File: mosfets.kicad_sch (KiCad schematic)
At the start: 25 parts, among them IC2 IRFR9014PBF, J4 Screw_Terminal_01x02, J5 Screw_Terminal_01x02, J6 Screw_Terminal_01x02, J7 Screw_Terminal_01x02, J8 Screw_Terminal_01x02, J9 Screw_Terminal_01x02, Q1 IRLML6244, Q2 IRLML6244, Q3 IRLML6244, Q4 IRLML6244, Q5 IRLML6244, Q6 IRLML6244

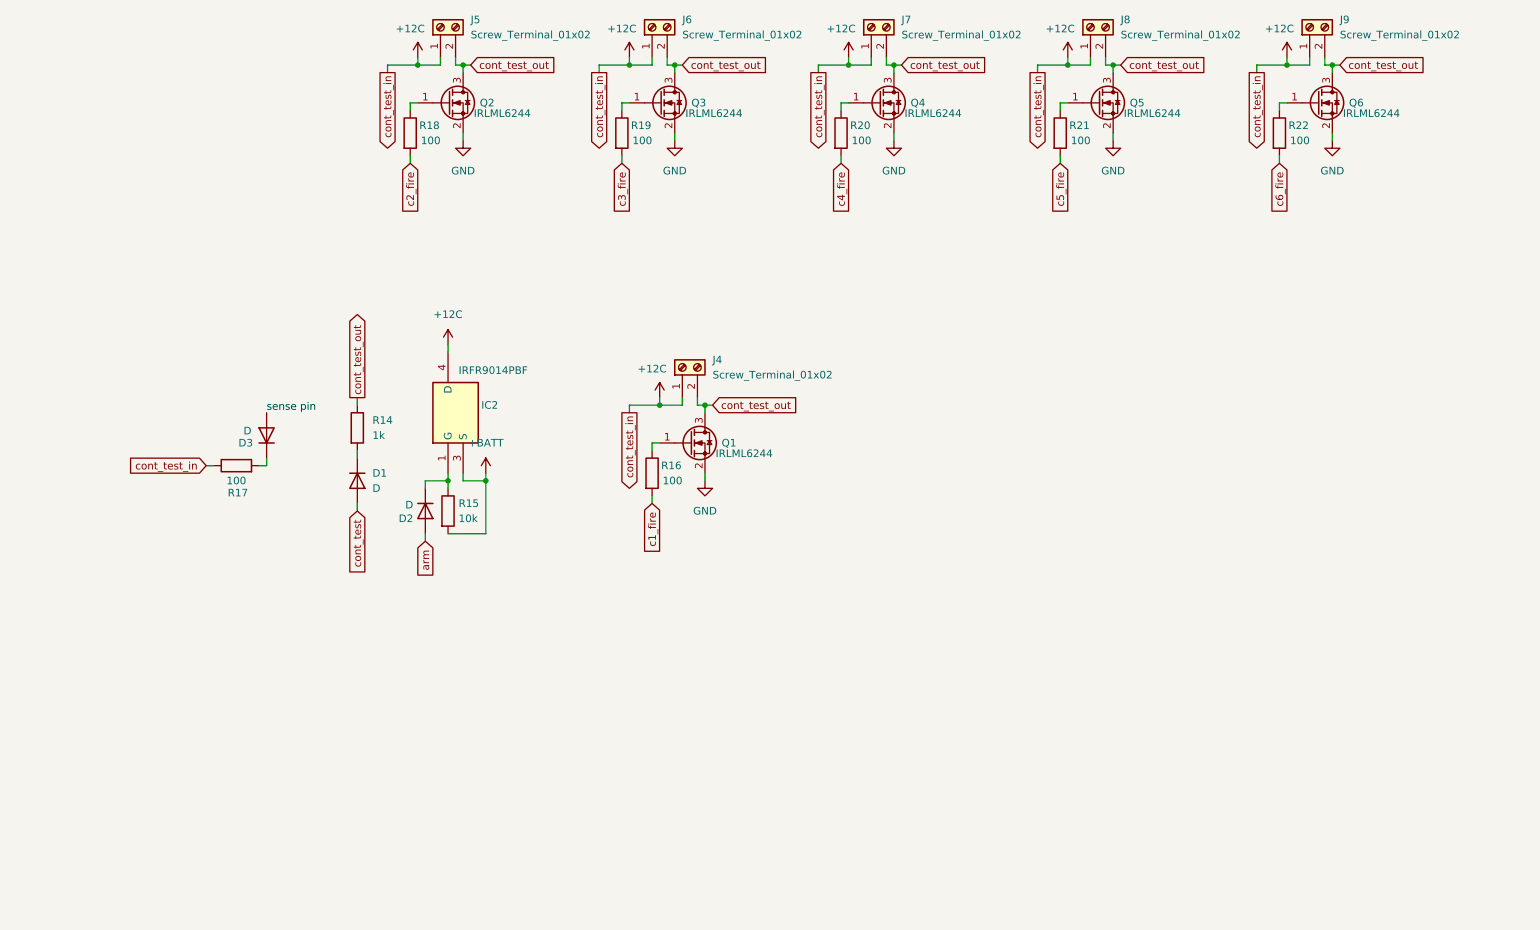
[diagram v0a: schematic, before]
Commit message: mosfet schematic done I hope
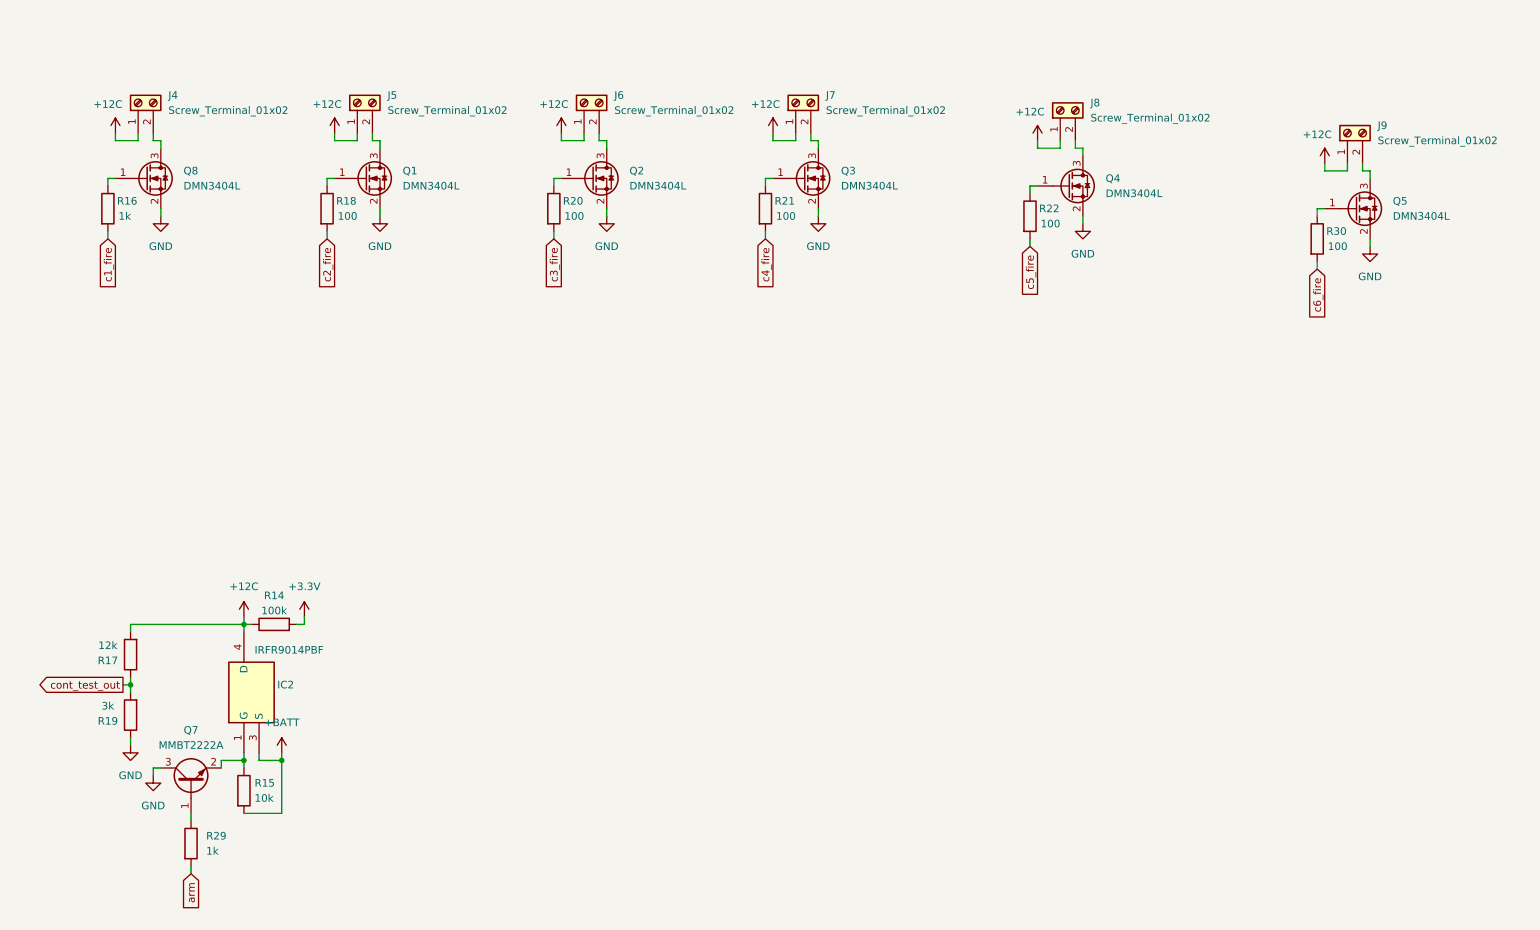
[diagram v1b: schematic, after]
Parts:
- removed D1, D2, D3: D, Diode_SMD:D_0603_1608Metric, symbol Device:D
- removed Q1, Q2, Q3, Q4, Q5, Q6: IRLML6244, Package_TO_SOT_SMD:SOT-23, symbol Transistor_FET:IRLML6244
- added Q1, Q2, Q3, Q4, Q5, Q8: DMN3404L, Package_TO_SOT_SMD:SOT-23, symbol Transistor_FET:DMN3404L
- added Q7: MMBT2222A, Package_TO_SOT_SMD:SOT-23, symbol Transistor_BJT:MMBT2222A
- added R29: 1k, Resistor_SMD:R_0402_1005Metric, symbol Device:R
- added R30: 100, Resistor_SMD:R_0603_1608Metric, symbol Device:R
- R14: value 1k -> 100k; footprint Resistor_SMD:R_0805_2012Metric -> Resistor_SMD:R_0603_1608Metric
- R16: value 100 -> 1k
- R17: value 100 -> 12k
- R19: value 100 -> 3k
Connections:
- net +12C: now also R14.1, R17.2; no longer R17.1
- net GND: now also R19.1, Q1.2 (S), Q2.2 (S), Q3.2 (S), Q4.2 (S), Q5.2 (S), Q7.3 (C), Q8.2 (S)
- net arm: now also R29.2
- net c3_fire: now also R20.2; no longer R19.2
- net c4_fire: now also R21.2; no longer R20.2
- net c5_fire: now also R22.2; no longer R21.2
- net c6_fire: now also R30.2; no longer R22.2
- net cont_test_out: now also R17.1, R19.2; no longer J4.2 (Pin_2), J5.2 (Pin_2), J6.2 (Pin_2), J7.2 (Pin_2), J8.2 (Pin_2), J9.2 (Pin_2), R14.1
- net at IC2.1 (G), R15.1: now also Q7.2 (E)
- net at R22.1: now also Q4.1 (G)
- net at R18.1: now also Q1.1 (G)
- net at R16.1: now also Q8.1 (G)
- net at R20.1: now also Q2.1 (G)
- net at R21.1: now also Q3.1 (G)
- net +3.3V: now reaches R14.2
- new net: J7.2 (Pin_2), Q3.3 (D)
- new net: J4.2 (Pin_2), Q8.3 (D)
- new net: Q7.1 (B), R29.1
- new net: J8.2 (Pin_2), Q4.3 (D)
- new net: J5.2 (Pin_2), Q1.3 (D)
- new net: J9.2 (Pin_2), Q5.3 (D)
- new net: Q5.1 (G), R30.1
- new net: J6.2 (Pin_2), Q2.3 (D)
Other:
- moved on the sheet: IC2, J4, J5, R15, R16, R18
